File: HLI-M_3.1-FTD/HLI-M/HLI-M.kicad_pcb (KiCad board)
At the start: 2 copper layers, 124.2 x 84.7 mm, 119 parts, among them CON1 , CON2 USB_B, CON3 , CON4 Connector_Adapter, CON5 Connector_Audio, CON6 Conn_01x15, CON7 Conn_01x09, CON8 CR123A, Q1 IRLML5103, Q2 BC817, Q3 BC817, Q4 BSS84, Q5 BSS84, Q6 BSS84, Q7 BSS84, U1 PIC24HJ64GP206-I_PT, U10 24AA02-OT, U10-A SOIC-8_3.9x4.9mm_P1.27mm, U11 ULN2003, U12 ULN2003, U13 ULN2003, U2 SOIC-8_3.9x4.9mm_P1.27mm, U2-A DFN-8-1EP_6x5mm_P1.27mm_EP2x2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, U3 MAX3232, U4 TPS7A0533PDBV, U5 TPS7A0533PDBV, U6 VSON-10-1EP_3x3mm_P0.5mm_EP1.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, U8 FT232RL, U9 SOIC-8_3.9x4.9mm_P1.27mm, Y1 Crystal_32KHz, Y2 Crystal_20MHz

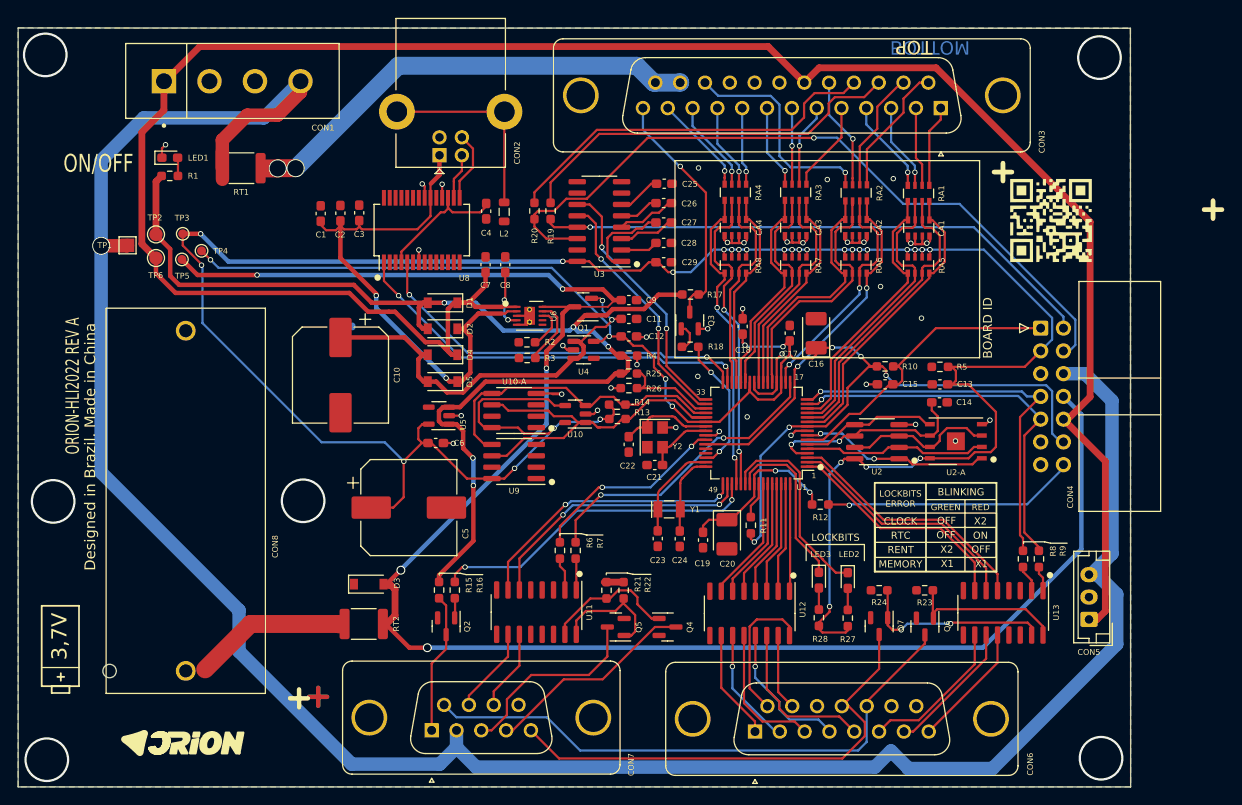
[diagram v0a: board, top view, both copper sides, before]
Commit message: att
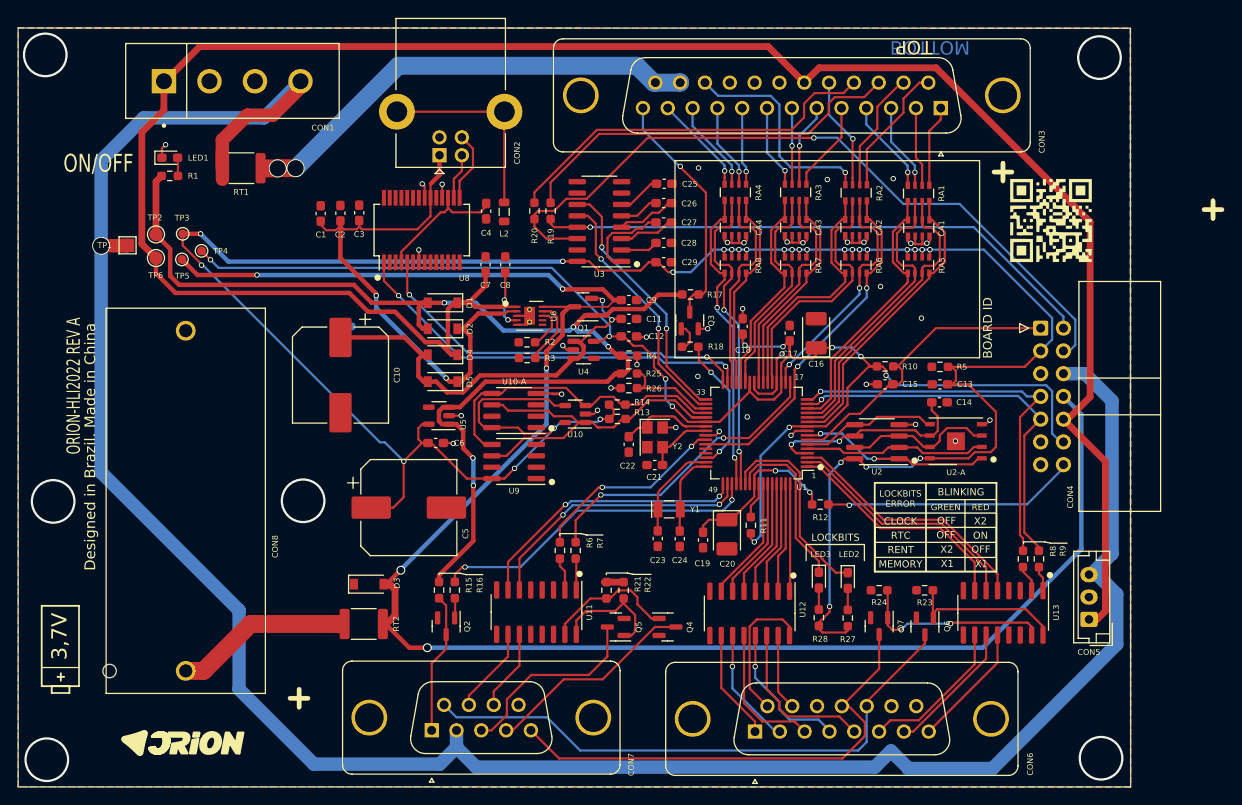
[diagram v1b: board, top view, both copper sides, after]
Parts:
- moved G*** 8.97 mm to (152.2, 87.7)
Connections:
- CON8 pad N: (no net) -> 0
- CON8 pad P: (no net) -> Net-(CON8-Pad1)
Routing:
- net +3V3: track 293.1 -> 289.4 mm
- net Net-(CON8-Pad1): track 17.1 -> 19.3 mm
- net +12V: track 261.9 -> 264.0 mm
